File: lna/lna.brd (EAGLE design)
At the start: 23 x 8.1 mm, 15 parts, among them U1 PSA4-5043, U4 MCP5301

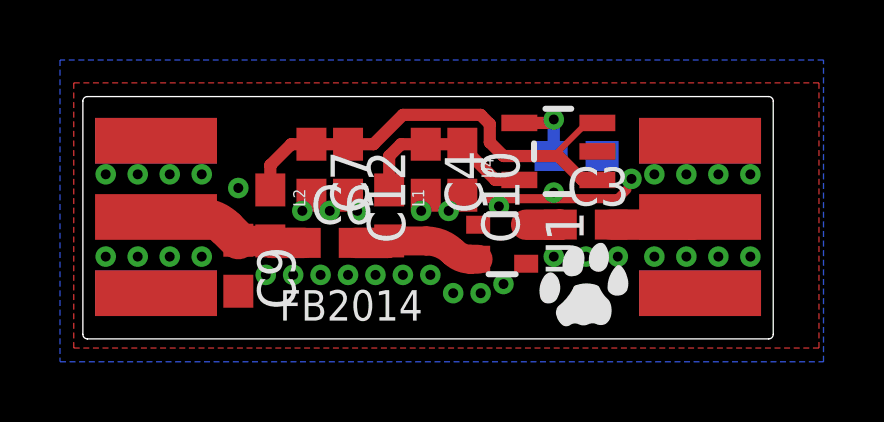
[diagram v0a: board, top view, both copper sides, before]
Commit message: r1
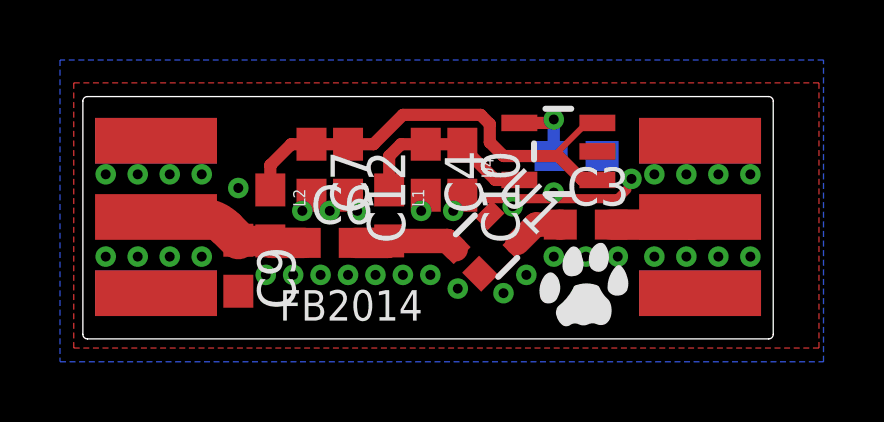
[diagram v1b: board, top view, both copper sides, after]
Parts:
- moved U1 0.52 mm to (13.5, 3.09), turned to 315 degrees
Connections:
- net GND: now also U1.2, U1.4; no longer U1.1, U1.3
- net N$2: now also U1.3; no longer U1.4
- net N$3: now also U1.1; no longer U1.2
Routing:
- net N$3: track 4.24 -> 3.49 mm
- net N$2: track 1.14 -> 1.69 mm
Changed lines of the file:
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@@
 <layer number="27" name="tValues" color="7" fill="1" visible="no" active="yes"/>
 <layer number="28" name="bValues" color="7" fill="1" visible="no" active="yes"/>
-<layer number="29" name="tStop" color="7" fill="3" visible="no" active="yes"/>
+<layer number="29" name="tStop" color="7" fill="3" visible="yes" active="yes"/>
 <layer number="30" name="bStop" color="7" fill="6" visible="no" active="yes"/>
 <layer number="31" name="tCream" color="7" fill="4" visible="no" active="yes"/>
@@
 <element name="J$1" library="SparkFun-Connectors" package="SMA-EDGE" value="SMA_EDGE" x="2.4384" y="1.524" rot="R90"/>
 <element name="J$2" library="SparkFun-Connectors" package="SMA-EDGE" value="SMA_EDGE" x="20.574" y="1.524" rot="R90"/>
-<element name="U1" library="balto" package="SOT343R" value="PSA4-5043" x="13.9761625" y="3.1557625" rot="R270"/>
+<element name="U1" library="balto" package="SOT343R" value="PSA4-5043" x="13.455834375" y="3.0926375" rot="R315"/>
 <element name="L1" library="SparkFun-Passives" package="0603" value="200n" x="10.2108" y="4.1148" rot="R270"/>
 <element name="C4" library="rcl" package="C0603" value="10n" x="11.43" y="5.6388" rot="R270"/>
@@
 <contactref element="C11" pad="2"/>
 <contactref element="C12" pad="2"/>
-<contactref element="U1" pad="1"/>
-<contactref element="U1" pad="3"/>
+<contactref element="U1" pad="2"/>
+<contactref element="U1" pad="4"/>
 <contactref element="C4" pad="2"/>
 <contactref element="C7" pad="2"/>
@@
 <via x="9.144" y="4.2672" extent="1-16" drill="0.3302"/>
 <via x="11.2776" y="4.2672" extent="1-16" drill="0.3302"/>
-<via x="12.192" y="4.2672" extent="1-16" drill="0.3302"/>
+<via x="12.3444" y="4.2672" extent="1-16" drill="0.3302"/>
 <via x="5.1816" y="5.0292" extent="1-16" drill="0.3302"/>
 <via x="6.096" y="2.1336" extent="1-16" drill="0.3302"/>
@@
 <via x="10.668" y="2.1336" extent="1-16" drill="0.3302"/>
 <via x="11.5824" y="2.1336" extent="1-16" drill="0.3302"/>
-<via x="14.0208" y="1.8288" extent="1-16" drill="0.3302"/>
-<via x="13.8684" y="4.4196" extent="1-16" drill="0.3302"/>
+<via x="14.7828" y="2.1336" extent="1-16" drill="0.3302"/>
+<via x="14.3256" y="4.4196" extent="1-16" drill="0.3302"/>
 <via x="15.6972" y="2.7432" extent="1-16" drill="0.3302"/>
 <via x="16.764" y="2.7432" extent="1-16" drill="0.3302"/>
@@
 <wire x1="13.4112" y1="4.6736" x2="17.8308" y2="4.6736" width="0.3048" layer="1"/>
 <wire x1="17.8308" y1="4.6736" x2="18.1356" y2="4.9784" width="0.3048" layer="1"/>
-<via x="12.3444" y="1.524" extent="1-16" drill="0.3302"/>
-<via x="13.2588" y="1.524" extent="1-16" drill="0.3302"/>
+<via x="12.4968" y="1.6764" extent="1-16" drill="0.3302"/>
+<via x="14.0208" y="1.524" extent="1-16" drill="0.3302"/>
 <via x="18.288" y="5.334" extent="1-16" drill="0.3302"/>
 </signal>
@@
 <signal name="N$2">
 <contactref element="C3" pad="1"/>
-<contactref element="U1" pad="4"/>
-<wire x1="14.7761625" y1="3.8057625" x2="15.9097625" y2="3.8057625" width="1.016" layer="1"/>
+<contactref element="U1" pad="3"/>
 <wire x1="15.9097625" y1="3.8057625" x2="15.914" y2="3.81" width="1.016" layer="1"/>
+<wire x1="15.914" y1="3.81" x2="15.092434375" y2="3.81" width="0.8128" layer="1"/>
+<wire x1="15.092434375" y1="3.81" x2="14.4811375" y2="3.198703125" width="0.8128" layer="1"/>
 </signal>
 <signal name="N$3">
@@
 <wire x1="9.0796" y1="3.2004" x2="10.1464" y2="3.2004" width="1.016" layer="1"/>
 <wire x1="10.1464" y1="3.2004" x2="10.2108" y2="3.2648" width="1.016" layer="1"/>
-<contactref element="U1" pad="2"/>
-<wire x1="10.2108" y1="3.2648" x2="11.44915" y2="3.2648" width="0.9652" layer="1"/>
-<wire x1="11.44915" y1="3.2648" x2="12.347175" y2="2.892825" width="0.9652" layer="1" curve="-45"/>
-<wire x1="12.347175" y1="2.892825" x2="12.91949375" y2="2.6557625" width="0.9652" layer="1" curve="45"/>
-<wire x1="12.91949375" y1="2.6557625" x2="13.1761625" y2="2.6557625" width="0.9652" layer="1"/>
+<contactref element="U1" pad="1"/>
+<wire x1="10.2108" y1="3.2648" x2="12.152296875" y2="3.2648" width="0.8128" layer="1"/>
+<wire x1="12.152296875" y1="3.2648" x2="12.430528125" y2="2.98656875" width="0.8128" layer="1"/>
 </signal>
 <signal name="N$9">
